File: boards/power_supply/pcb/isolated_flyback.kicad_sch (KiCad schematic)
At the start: 19 parts, among them T701 150u

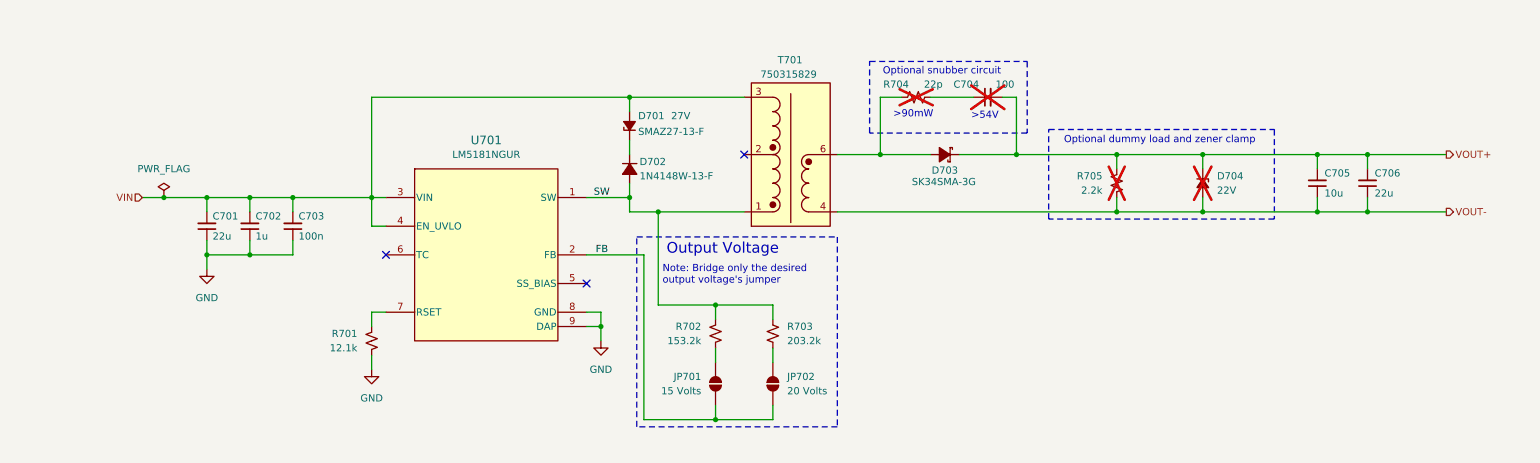
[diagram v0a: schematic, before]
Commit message: starting psu layout
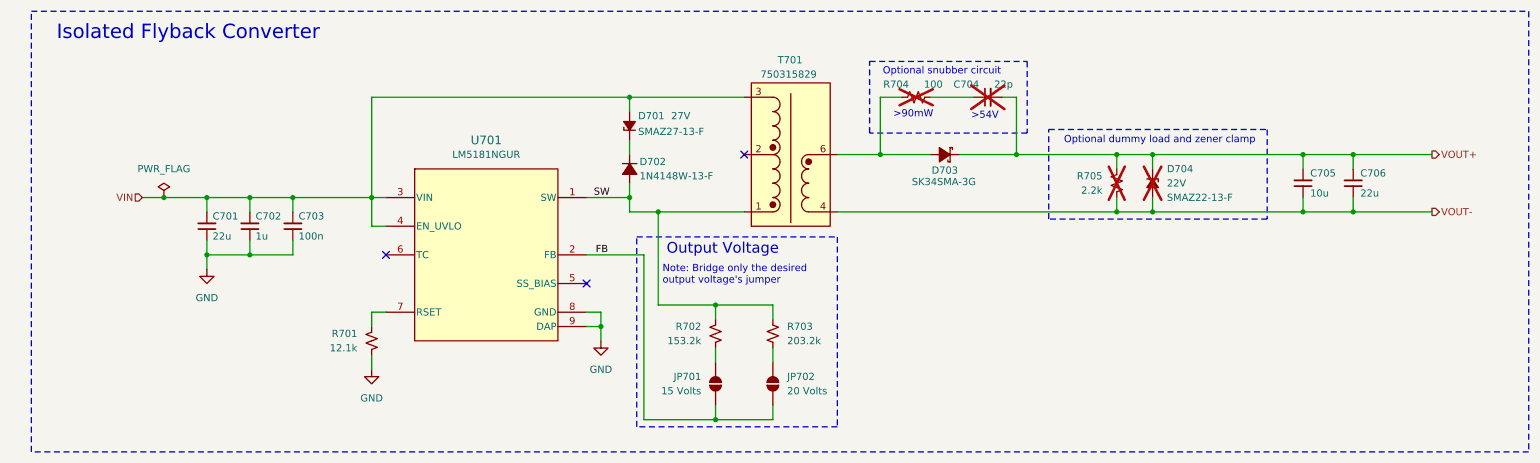
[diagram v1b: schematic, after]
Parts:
- removed D704: 22V, symbol Device:D_Zener_Small_Filled
- added D704: 22V, SMAZ22-13-F:SMAZ22-13-F, symbol SMAZ22-13-F:SMAZ22-13-F
- C701, C706: footprint (none) -> Capacitor_SMD:C_1206_3216Metric
- C702, C703: footprint (none) -> Capacitor_SMD:C_0603_1608Metric
- C704: value 100 -> 22p; footprint (none) -> Capacitor_SMD:C_0603_1608Metric
- C705: footprint (none) -> Capacitor_SMD:C_0805_2012Metric
- D701: footprint (none) -> SMAZ27-13-F:SMAZ27-13-F
- JP701, JP702: footprint (none) -> Jumper:SolderJumper-2_P1.3mm_Open_RoundedPad1.0x1.5mm
- R701, R702, R703, R705: footprint (none) -> Resistor_SMD:R_0603_1608Metric
- R704: value 22p -> 100; footprint (none) -> Resistor_SMD:R_0603_1608Metric
- T701: footprint (none) -> 750315829:750315829
- U701: footprint NGU0008C-IPC_A -> LM5181NGUR:NGU0008C-IPC_A
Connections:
- net VOUT+: now also D704.1 (K)
- net VOUT-: now also D704.2 (A)
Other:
- note added: "Isolated Flyback Converter"
- moved on the sheet: C705, C706
